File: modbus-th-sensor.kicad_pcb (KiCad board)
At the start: 2 copper layers, 42 parts, among them J1 Screw Terminal, J2 FTDI Serial, J3 ICSP, Q1 AO3401A, SW2 TERM, SW3 Node ID, U1 ATmega328P-A, U2 SHT4x, U3 SP3485EN, U5 AP63203WU, Y1 8MHz

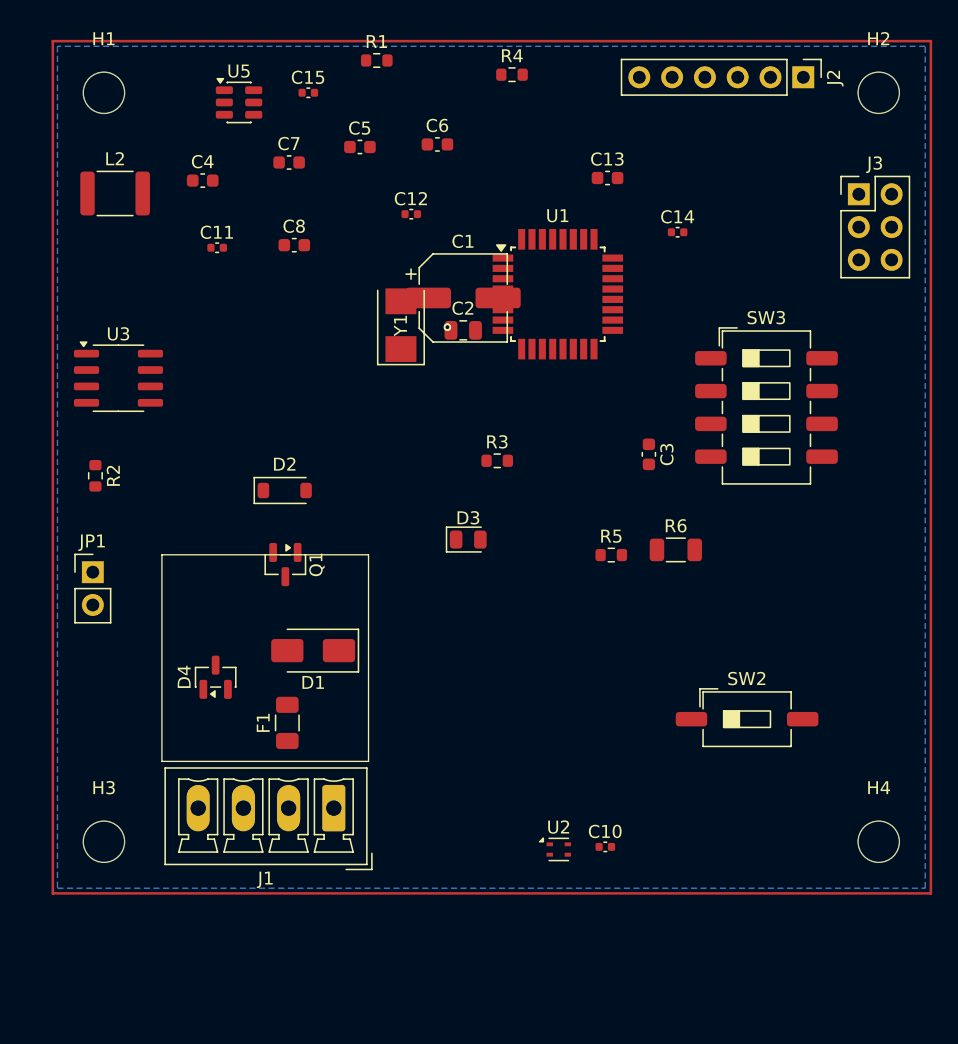
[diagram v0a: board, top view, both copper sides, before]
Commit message: Finished routing main board
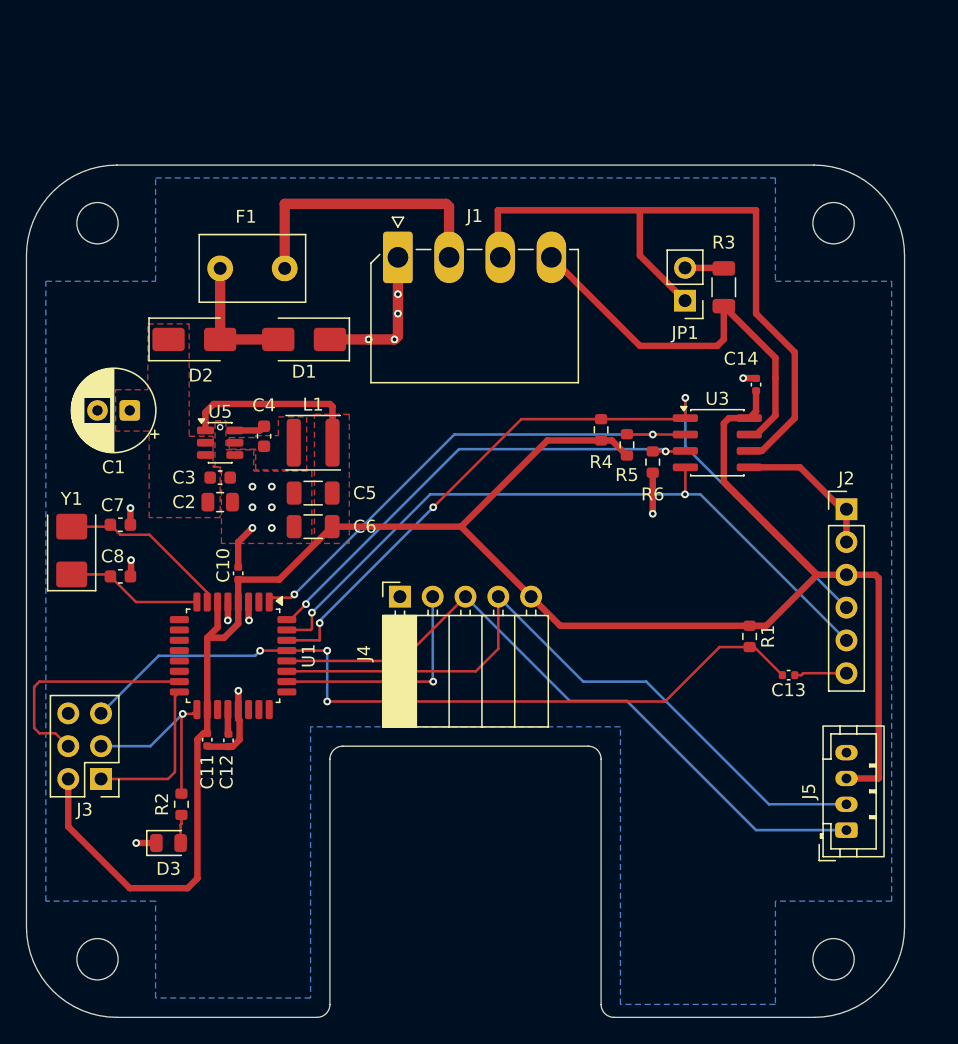
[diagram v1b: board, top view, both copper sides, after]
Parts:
- removed C15: 0.1uF, Capacitor_SMD:C_0402_1005Metric
- removed D4: SM712, Package_TO_SOT_SMD:SOT-23
- removed Q1: AO3401A, Package_TO_SOT_SMD:SOT-23
- removed the R1 at (143.1, 58.9)
- removed SW2: TERM, Button_Switch_SMD:SW_DIP_SPSTx01_Slide_6.7x4.1mm_W8.61mm_P2.54mm_LowProfile
- removed SW3: Node ID, Button_Switch_SMD:SW_DIP_SPSTx04_Slide_6.7x11.72mm_W8.61mm_P2.54mm_LowProfile
- removed U2: SHT4x, Sensor_Humidity:Sensirion_DFN-4_1.5x1.5mm_P0.8mm_SHT4x_NoCentralPad
- added J4: Sensor Board, Connector_PinSocket_2.54mm:PinSocket_1x05_P2.54mm_Horizontal, F.Cu at (144.9, 100.4)
- added J5: I2C, Connector_JST:JST_PH_B4B-PH-K_1x04_P2.00mm_Vertical, F.Cu at (179.5, 118.5)
- added R6: 10K, Resistor_SMD:R_0603_1608Metric, F.Cu at (164.5, 90.0)
- C1: footprint Capacitor_SMD:CP_Elec_6.3x5.8 -> Capacitor_THT:CP_Radial_D6.3mm_P2.50mm
- C13: footprint Capacitor_SMD:C_0603_1608Metric -> Capacitor_SMD:C_0402_1005Metric
- C5, C6: footprint Capacitor_SMD:C_0603_1608Metric -> Capacitor_SMD:C_1206_3216Metric
- D1: value SMAJ18CA -> SMAJ24CA
- D2: value 10V -> SS210; footprint Diode_SMD:D_SOD-123 -> Diode_SMD:D_SMA
- F1: value 0.75A -> 0.5A; footprint Fuse:Fuse_1206_3216Metric -> Capacitor_THT:C_Disc_D8.0mm_W5.0mm_P5.00mm
- J1: footprint Connector_Phoenix_MC:PhoenixContact_MCV_1,5_4-G-3.5_1x04_P3.50mm_Vertical -> Kefa HT396:Kefa_HT396R-3.96-04P_1x04_P3.96mm_Horizontal
- JP1: value Jumper_2_Open -> Terminate
- L1: renamed from L2; footprint Inductor_SMD:L_1812_4532Metric -> Inductor_SMD:L_Sunlord_SWPA4030S
- R2: renamed from R3; value 330R -> 1K
- R4, R5: value 4.7k -> 10K
- U3: value SP3485EN -> THVD2410DR
- moved J3 74.1 mm to (121.8, 114.5), turned to 180 degrees
- moved R1 52.2 mm to (172.0, 103.5)
- moved JP1 50.4 mm to (167.0, 77.5), turned to 180 degrees
- moved U3 46.6 mm to (169.5, 88.5)
- moved C12 43.1 mm to (131.6, 111.6), turned to -90 degrees
- moved J1 42.9 mm to (144.8, 74.1), turned to 0 degrees
- moved C13 41.0 mm to (175.0, 106.5), turned to 180 degrees
- moved C11 38.1 mm to (130.0, 111.5), turned to -90 degrees
- moved U1 37.6 mm to (132.0, 105.0), turned to -90 degrees
- moved R2 36.1 mm to (128.0, 116.5), turned to -90 degrees
- moved C10 35.5 mm to (132.4, 98.6), turned to 90 degrees
- moved F1 35.2 mm to (136.0, 75.0), turned to 180 degrees
- moved J2 33.6 mm to (179.5, 93.7), turned to 0 degrees
- moved C3 33.2 mm to (131.0, 91.2), turned to 0 degrees
- moved D3 33.0 mm to (127.0, 119.5)
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- renumbered R2 to R1, R6 to R3
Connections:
- net Net-(D2-K) renamed /VIN_PROT
- C13 pad 1: Net-(J2-Pin_1) -> Net-(J2-Pin_6)
- D1 pad 2: Net-(D1-A2) -> /VIN_FUSED
- D2 pad 2: Net-(D2-A) -> /VIN_FUSED
- F1 pad 2: Net-(D1-A2) -> /VIN_FUSED
- J2 pad 1: Net-(J2-Pin_1) -> GND
- J2 pad 2: RXD -> GND
- J2 pad 3: TXD -> +3.3V
- J2 pad 4: +3.3V -> RXI
- J2 pad 5: GND -> TXO
- J2 pad 6: GND -> Net-(J2-Pin_6)
- JP1 pad 1: Net-(JP1-A) -> A
- JP1 pad 2: A -> Net-(JP1-B)
- R3 pad 2: Net-(R6-Pad2) -> Net-(JP1-B)
- R4 pad 2: SDA -> RXI
- R5 pad 2: SCL -> RXEN
- U1 pad 1: TXEN -> RXEN
- U1 pad 10: ID2 -> unconnected-(U1-PD6-Pad10)
- U1 pad 11: ID3 -> unconnected-(U1-PD7-Pad11)
- U1 pad 2: ID0 -> unconnected-(U1-PD4-Pad2)
- U1 pad 26: unconnected-(U1-PC3-Pad26) -> INT
- U1 pad 30: RXD -> RXI
- U1 pad 31: TXD -> TXO
- U1 pad 32: RXEN -> TXEN
- U1 pad 9: ID1 -> unconnected-(U1-PD5-Pad9)
- U3 pad 1: RXD -> RXI
- U3 pad 4: TXD -> TXO
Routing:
- net +3.3V: track 0.00 -> 168.6 mm
- net RXI: track 0.00 -> 61.9 mm, vias 0 -> 3
- net RESET: track 0.00 -> 61.5 mm, vias 0 -> 3
- net TXO: track 0.00 -> 55.3 mm, vias 0 -> 2
- net SDA: track 0.00 -> 54.8 mm
- net A: track 0.00 -> 54.1 mm
- net SCL: track 0.00 -> 52.9 mm
- net GND: track 0.00 -> 44.1 mm, vias 0 -> 19
- net RXEN: track 0.00 -> 39.6 mm, vias 0 -> 2
- net TXEN: track 0.00 -> 37.5 mm, vias 0 -> 2
- net B: track 0.00 -> 33.2 mm
- net Vin: track 0.00 -> 21.7 mm
- net INT: track 0.00 -> 17.9 mm, vias 0 -> 1
- net SDO: track 0.00 -> 17.8 mm
- net SCK: track 0.00 -> 14.8 mm, vias 0 -> 1
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- added copper zone on F.Cu, net +3.3V
- added copper zone on F.Cu, net /VIN_PROT
- added copper zone on F.Cu, net GND
- added copper zone on F.Cu, net Net-(U5-SW)
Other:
- board outline added: 68 x 66 mm
- board text added: "MCU"
- board text added: "Power"
- board text added: "RS-485"
- board text added: "Sensor board"
